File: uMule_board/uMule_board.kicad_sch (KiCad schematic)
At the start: 0 parts

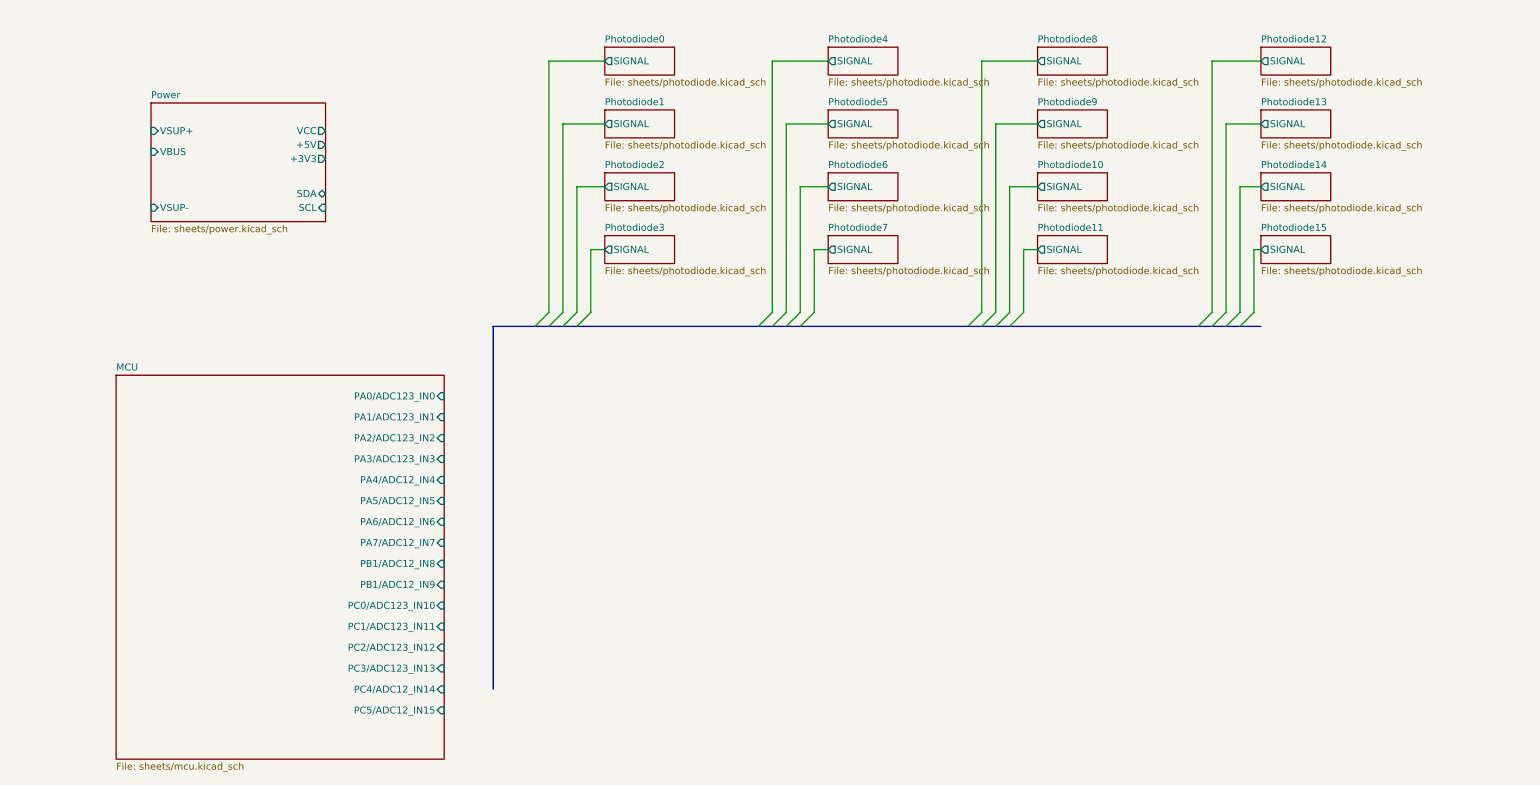
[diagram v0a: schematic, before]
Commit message: Some calculations were made. Photodiode, amplifier and main procesor are chosen
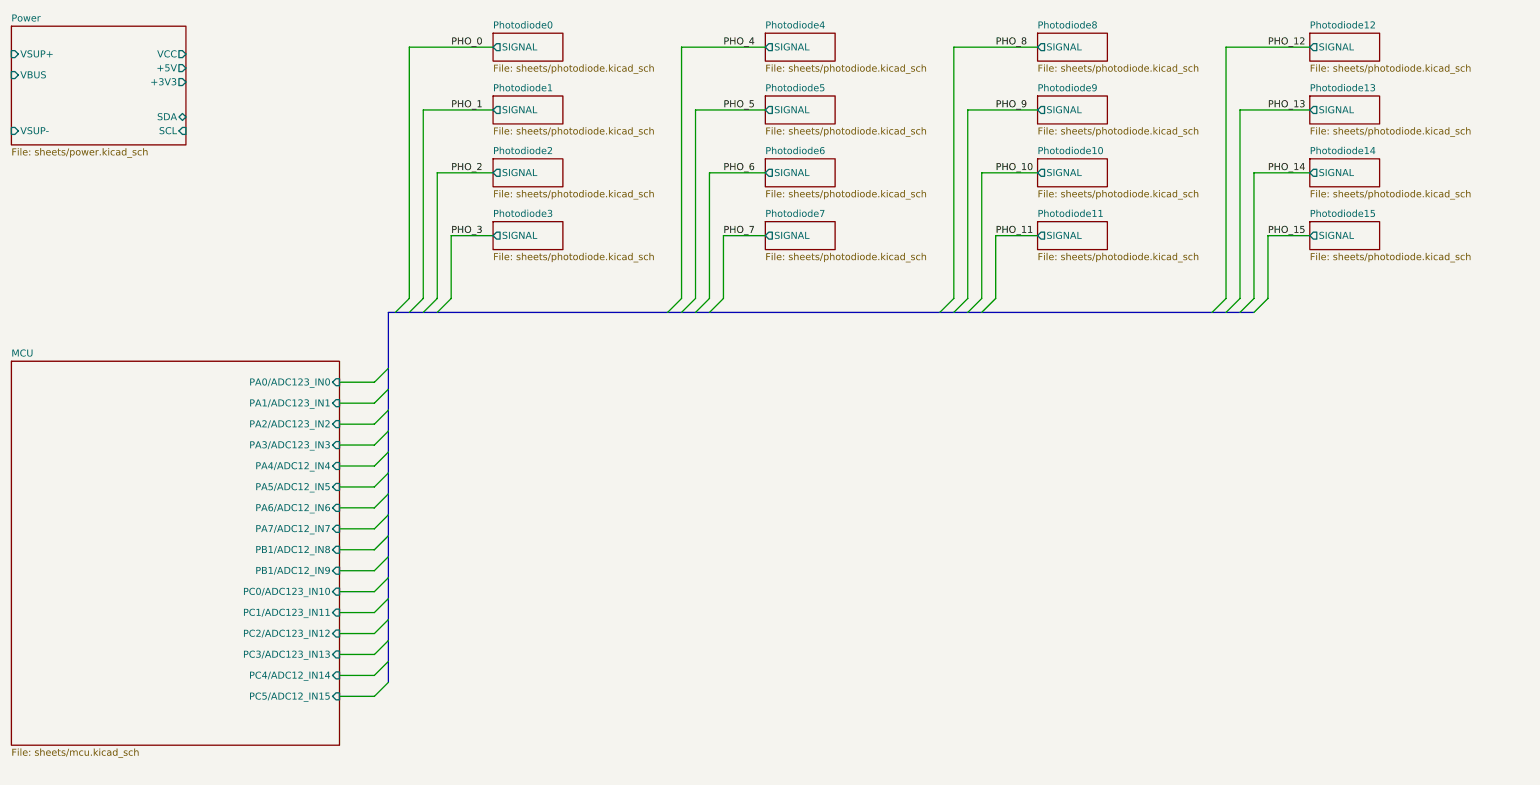
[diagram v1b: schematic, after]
